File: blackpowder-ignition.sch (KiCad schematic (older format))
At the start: 7 parts, among them J1 CAS_stacking, J8 Conn_01x02, U1 TCA9555PWR

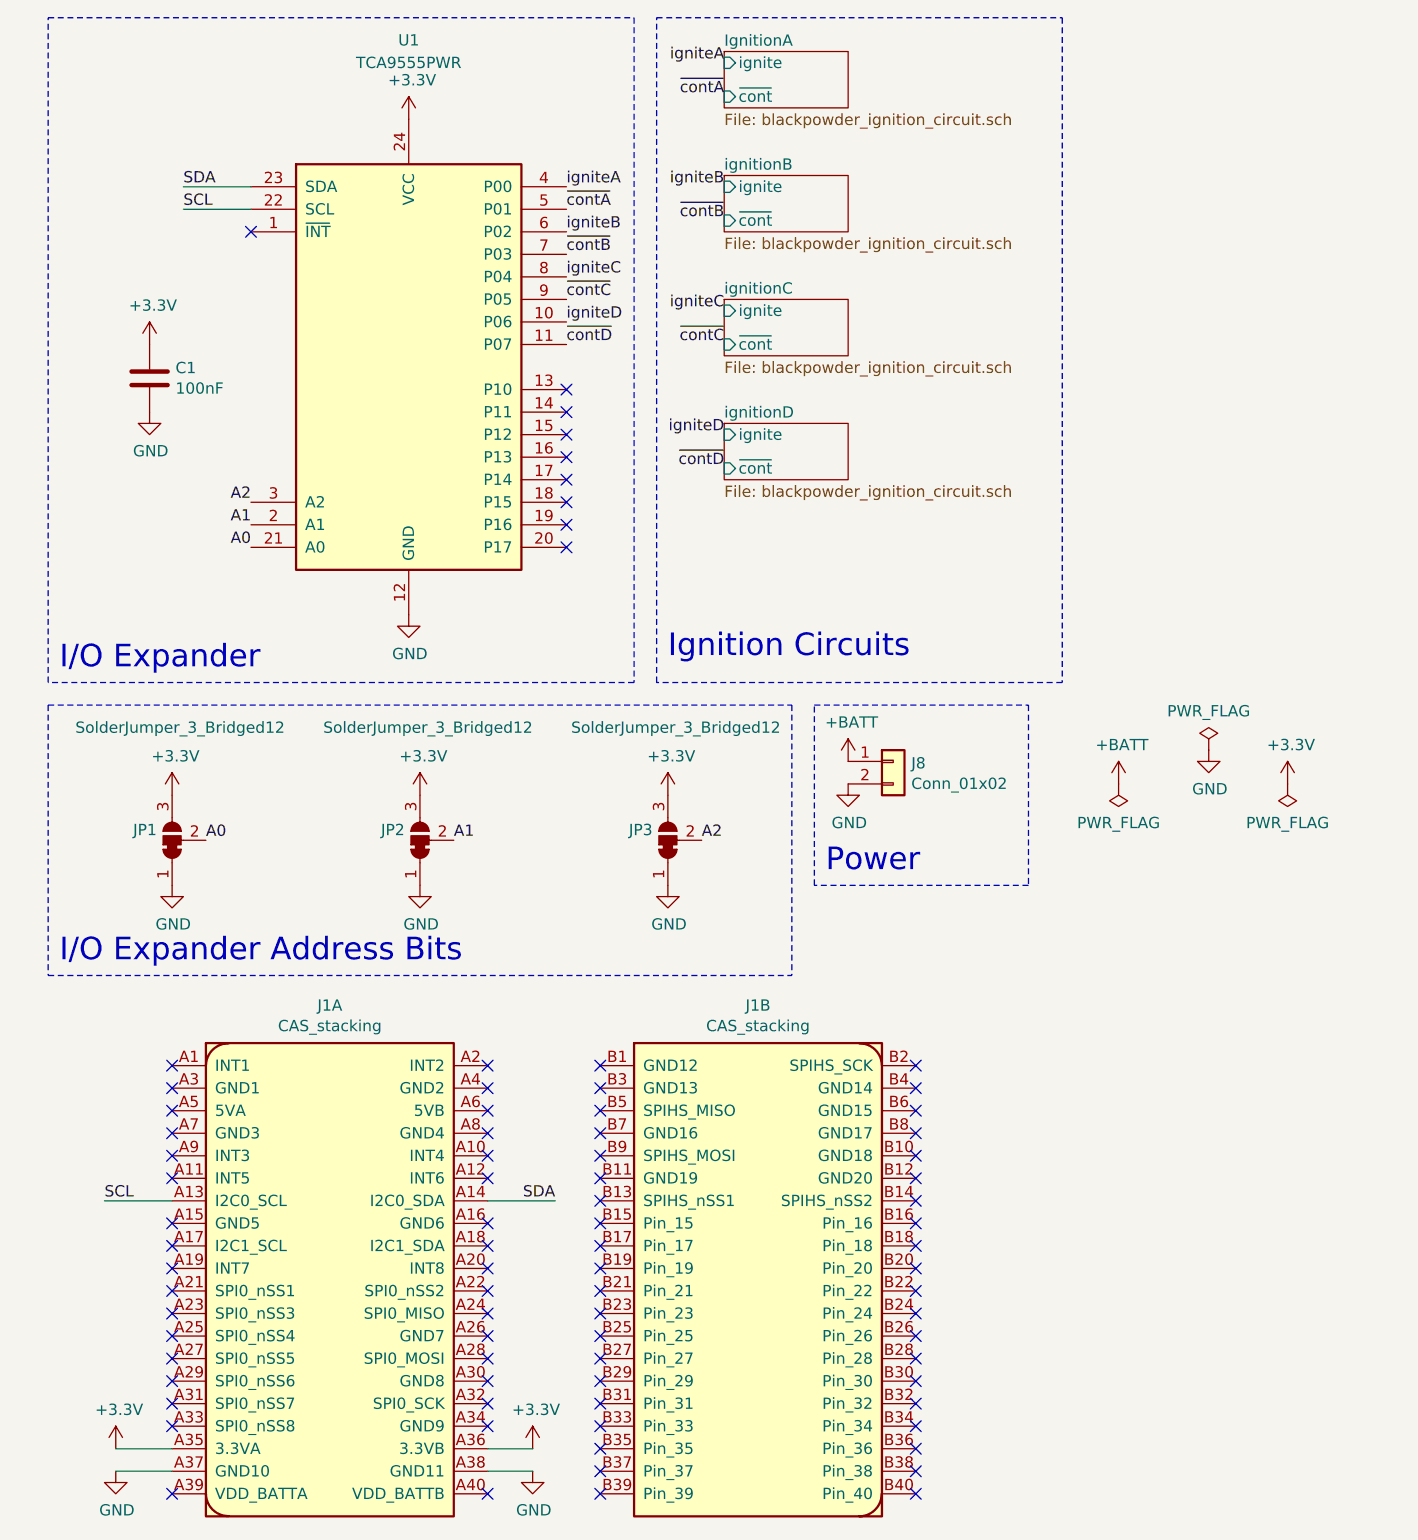
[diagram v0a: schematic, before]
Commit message: most functionality
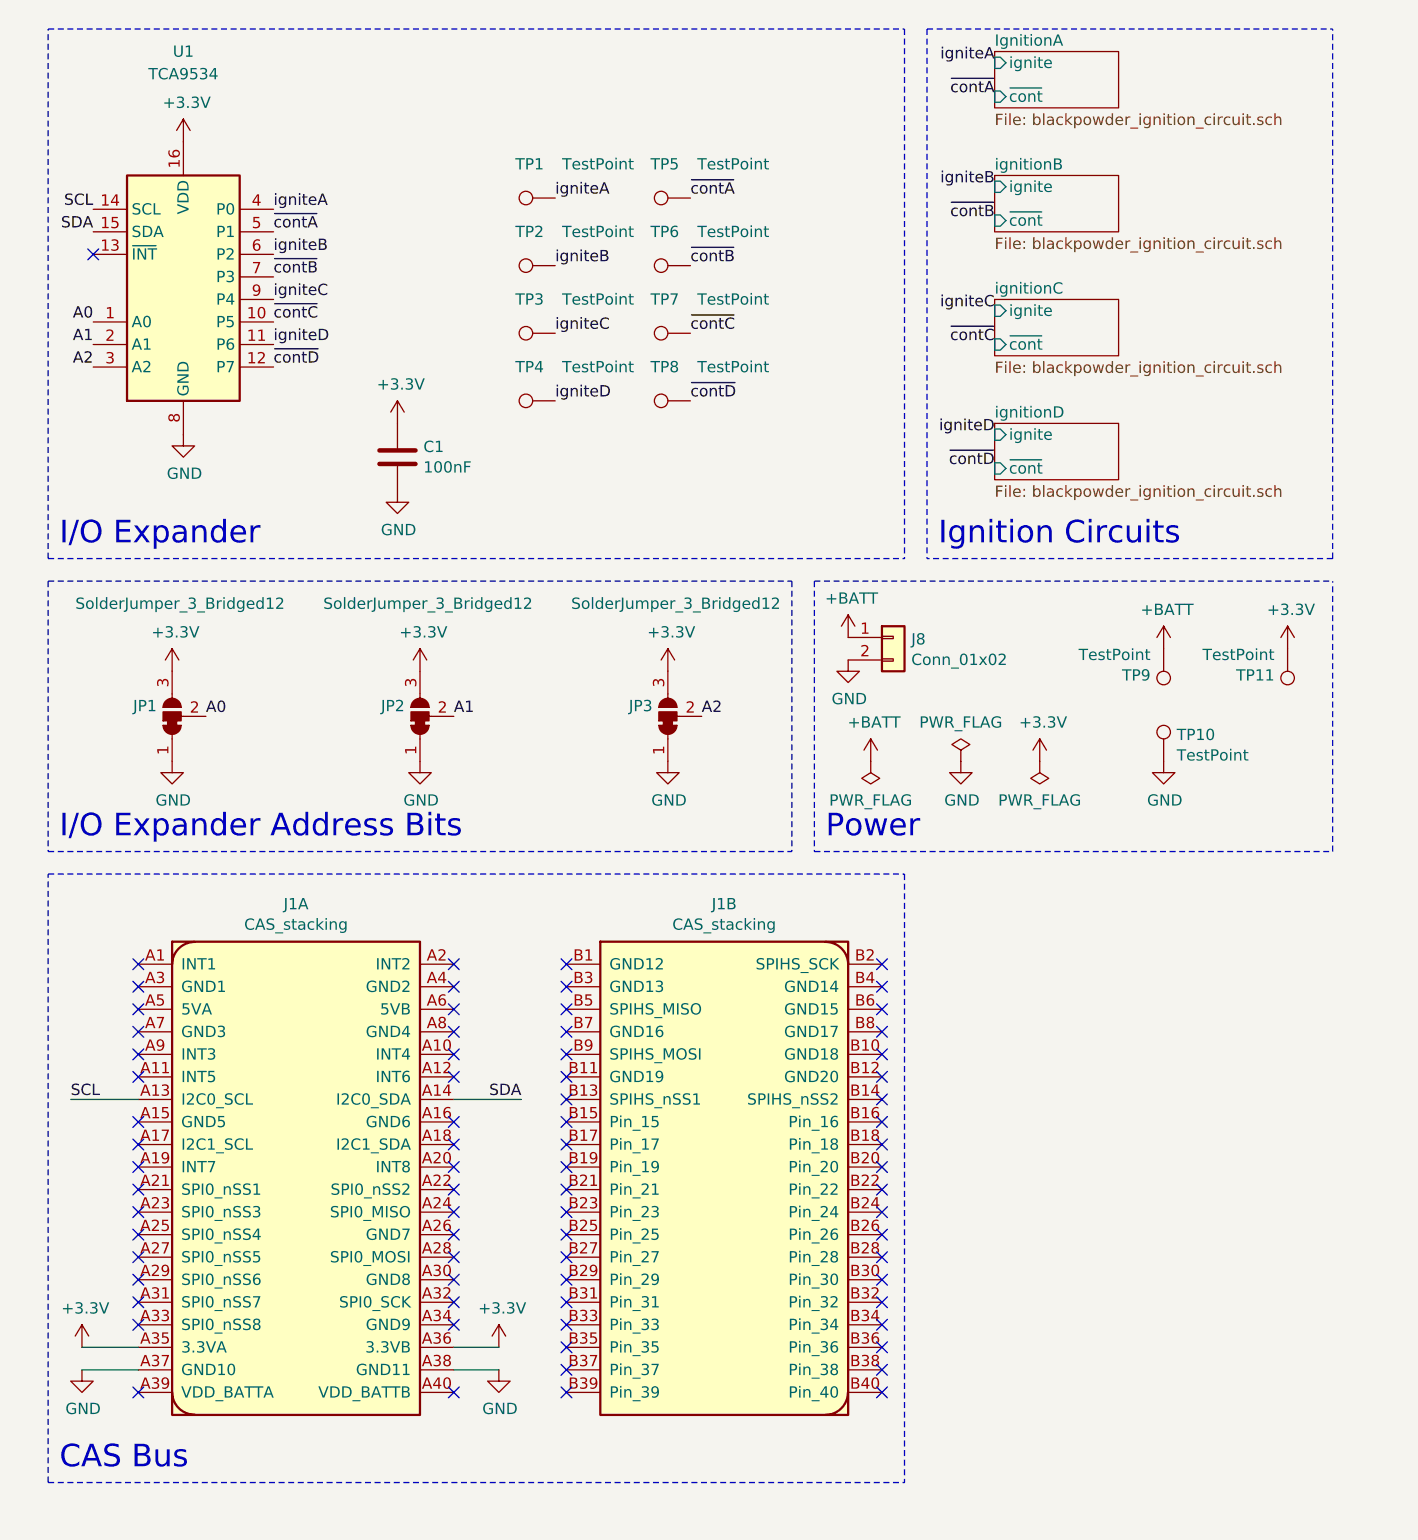
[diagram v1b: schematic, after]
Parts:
- removed U1: TCA9555PWR, Package_SO:TSSOP-24_4.4x7.8mm_P0.65mm, symbol Interface_Expansion:TCA9555PWR
- added TP1, TP2, TP3, TP4, TP5, TP6, TP7, TP8: TestPoint, star-common-lib:TestPoint_Keystone_5117_Miniature, symbol Connector:TestPoint
- added TP10, TP11, TP9: TestPoint, star-common-lib:TestPoint_Keystone_5000_Miniature, symbol Connector:TestPoint
- added U1: TCA9534, Package_SO:TSSOP-16_4.4x5mm_P0.65mm, symbol Interface_Expansion:TCA9534
- J8: footprint Connector_Molex:Molex_Mini-Fit_Jr_5569-02A2_2x01_P4.20mm_Horizontal -> star-common-lib:Molex_Mini-Fit_Jr_5569-02A2_2x01_P4.20mm_Horizontal
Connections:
- net +3V3: now also TP11.1, U1.16 (VDD)
- net +BATT: now also TP9.1
- net A0: now also U1.1 (A0)
- net A1: now also U1.2 (A1)
- net A2: now also U1.3 (A2)
- net GND: now also TP10.1, U1.8 (GND)
- net SCL: now also U1.14 (SCL)
- net SDA: now also U1.15 (SDA)
- net igniteA: now also TP1.1, U1.4 (P0)
- net igniteB: now also TP2.1, U1.6 (P2)
- net igniteC: now also TP3.1, U1.9 (P4)
- net igniteD: now also TP4.1, U1.11 (P6)
- net ~contA~: now also TP5.1, U1.5 (P1)
- net ~contB~: now also TP6.1, U1.7 (P3)
- net ~contC~: now also TP7.1, U1.10 (P5)
- net ~contD~: now also TP8.1, U1.12 (P7)
- no-connect marks 83 -> 75
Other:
- note added: "CAS Bus"
- moved on the sheet: C1, J1A, J1B, J8, JP1, JP2, JP3
